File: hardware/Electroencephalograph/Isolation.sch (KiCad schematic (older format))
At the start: 17 parts, among them U4 THI3-0511, U5 ADUM2401BRWZ

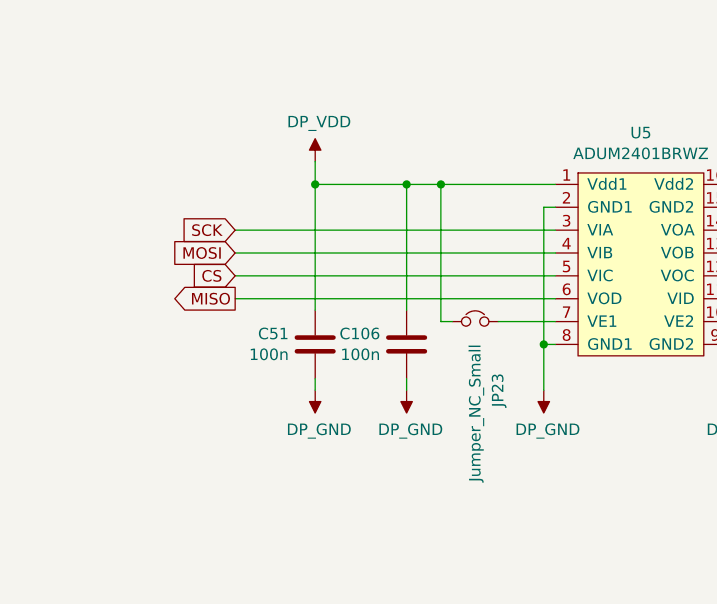
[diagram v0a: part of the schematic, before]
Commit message: further routing
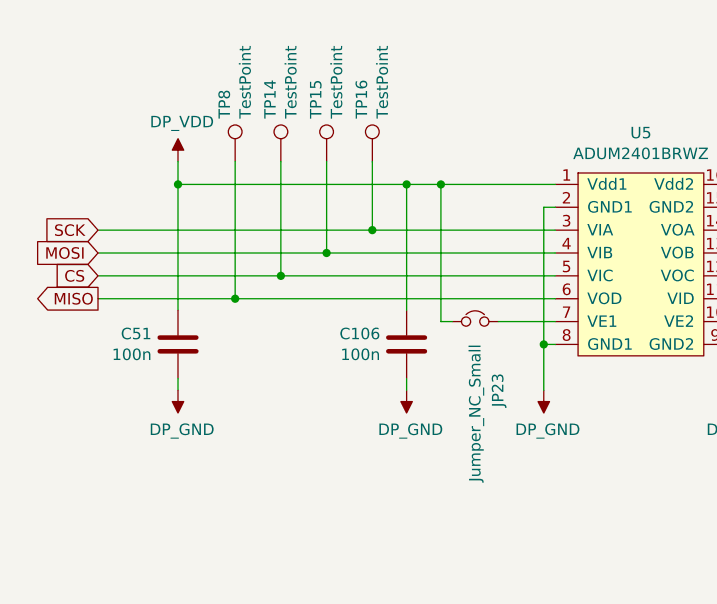
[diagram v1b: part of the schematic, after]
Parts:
- added TP14, TP15, TP16, TP8: TestPoint, TestPoint:TestPoint_Pad_D1.0mm, symbol Connector:TestPoint
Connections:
- net CS: now also TP14.1
- net MISO: now also TP8.1
- net MOSI: now also TP15.1
- net SCK: now also TP16.1
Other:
- moved on the sheet: C51
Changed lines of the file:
@@
 Wire Wire Line
 	3100 2600 3100 3200
-Text GLabel 1750 2700 0    50   Input ~ 0
+Text GLabel 1150 2700 0    50   Input ~ 0
 SCK
-Text GLabel 1750 2800 0    50   Input ~ 0
+Text GLabel 1150 2800 0    50   Input ~ 0
 MOSI
-Text GLabel 1750 2900 0    50   Input ~ 0
+Text GLabel 1150 2900 0    50   Input ~ 0
 CS
-Text GLabel 1750 3000 0    50   Output ~ 0
+Text GLabel 1150 3000 0    50   Output ~ 0
 MISO
 Wire Wire Line
-	3150 2700 1750 2700
-Wire Wire Line
-	3150 2800 1750 2800
-Wire Wire Line
-	3150 2900 1750 2900
-Wire Wire Line
-	3150 3000 1750 3000
-Connection ~ 2100 2500
-Wire Wire Line
-	2100 2500 2100 2400
-Wire Wire Line
-	2100 2500 2100 3050
+	3150 2700 2350 2700
+Wire Wire Line
+	3150 2800 2150 2800
+Wire Wire Line
+	3150 2900 1950 2900
+Connection ~ 1500 2500
+Wire Wire Line
+	1500 2500 1500 2400
+Wire Wire Line
+	1500 2500 1500 3050
 $Comp
 L Device:C C?
 U 1 1 5E028BA8
-P 2100 3200
+P 1500 3200
 AR Path="/5DF4CFF8/5E028BA8" Ref="C?"  Part="1"
 AR Path="/5DF61103/5E028BA8" Ref="C?"  Part="1"
 AR Path="/5DFE0AD6/5E028BA8" Ref="C51"  Part="1"
-F 0 "C51" H 2215 3246 50  0000 L CNN
-F 1 "100n" H 2215 3155 50  0000 L CNN
-F 2 "Capacitor_SMD:C_0402_1005Metric" H 2138 3050 50  0001 C CNN
-F 3 "~" H 2100 3200 50  0001 C CNN
-	1    2100 3200
+F 0 "C51" H 1615 3246 50  0000 L CNN
+F 1 "100n" H 1615 3155 50  0000 L CNN
+F 2 "Capacitor_SMD:C_0402_1005Metric" H 1538 3050 50  0001 C CNN
+F 3 "~" H 1500 3200 50  0001 C CNN
+	1    1500 3200
 	-1   0    0    -1
 $EndComp
@@
 L Electroencephalograph:DP_VDD #PWR101
 U 1 1 5E02F433
-P 2100 2400
-F 0 "#PWR101" H 2100 2525 50  0001 C CNN
-F 1 "DP_VDD" H 2117 2573 50  0000 C CNN
-F 2 "" H 2100 2525 50  0001 C CNN
-F 3 "" H 2100 2525 50  0001 C CNN
-	1    2100 2400
+P 1500 2400
+F 0 "#PWR101" H 1500 2525 50  0001 C CNN
+F 1 "DP_VDD" H 1517 2573 50  0000 C CNN
+F 2 "" H 1500 2525 50  0001 C CNN
+F 3 "" H 1500 2525 50  0001 C CNN
+	1    1500 2400
 	1    0    0    -1
 $EndComp
@@
 L Electroencephalograph:DP_GND #PWR102
 U 1 1 5E02EFAB
-P 2100 3400
-F 0 "#PWR102" H 2100 3425 50  0001 C CNN
-F 1 "DP_GND" H 2117 3227 50  0000 C CNN
-F 2 "" H 2100 3425 50  0001 C CNN
-F 3 "" H 2100 3425 50  0001 C CNN
-	1    2100 3400
+P 1500 3400
+F 0 "#PWR102" H 1500 3425 50  0001 C CNN
+F 1 "DP_GND" H 1517 3227 50  0000 C CNN
+F 2 "" H 1500 3425 50  0001 C CNN
+F 3 "" H 1500 3425 50  0001 C CNN
+	1    1500 3400
 	1    0    0    -1
 $EndComp
@@
 $EndComp
 Wire Wire Line
-	2100 3400 2100 3350
+	1500 3400 1500 3350
 Connection ~ 3100 3200
 Wire Wire Line
@@
 	2500 3050 2500 2500
 Wire Wire Line
-	2100 2500 2500 2500
+	1500 2500 2500 2500
 Connection ~ 2500 2500
 Wire Wire Line
@@
 Wire Wire Line
 	4650 2500 5050 2500
+$Comp
+L Connector:TestPoint TP?
+U 1 1 5E2E87E0
+P 2350 2400
+AR Path="/5DF61103/5E2E87E0" Ref="TP?"  Part="1"
+AR Path="/5E142744/5E2E87E0" Ref="TP?"  Part="1"
+AR Path="/5DFE0AD6/5E2E87E0" Ref="TP16"  Part="1"
+F 0 "TP16" V 2304 2588 50  0000 L CNN
+F 1 "TestPoint" V 2395 2588 50  0000 L CNN
+F 2 "TestPoint:TestPoint_Pad_D1.0mm" H 2550 2400 50  0001 C CNN
+F 3 "~" H 2550 2400 50  0001 C CNN
+	1    2350 2400
+	1    0    0    -1
+$EndComp
+$Comp
+L Connector:TestPoint TP?
+U 1 1 5E2E87E6
+P 2150 2400
+AR Path="/5DF61103/5E2E87E6" Ref="TP?"  Part="1"
+AR Path="/5E142744/5E2E87E6" Ref="TP?"  Part="1"
+AR Path="/5DFE0AD6/5E2E87E6" Ref="TP15"  Part="1"
+F 0 "TP15" V 2104 2588 50  0000 L CNN
+F 1 "TestPoint" V 2195 2588 50  0000 L CNN
+F 2 "TestPoint:TestPoint_Pad_D1.0mm" H 2350 2400 50  0001 C CNN
+F 3 "~" H 2350 2400 50  0001 C CNN
+	1    2150 2400
+	1    0    0    -1
+$EndComp
+$Comp
+L Connector:TestPoint TP?
+U 1 1 5E2E87EC
+P 1950 2400
+AR Path="/5DF61103/5E2E87EC" Ref="TP?"  Part="1"
+AR Path="/5E142744/5E2E87EC" Ref="TP?"  Part="1"
+AR Path="/5DFE0AD6/5E2E87EC" Ref="TP14"  Part="1"
+F 0 "TP14" V 1904 2588 50  0000 L CNN
+F 1 "TestPoint" V 1995 2588 50  0000 L CNN
+F 2 "TestPoint:TestPoint_Pad_D1.0mm" H 2150 2400 50  0001 C CNN
+F 3 "~" H 2150 2400 50  0001 C CNN
+	1    1950 2400
+	1    0    0    -1
+$EndComp
+$Comp
+L Connector:TestPoint TP?
+U 1 1 5E2E87F2
+P 1750 2400
+AR Path="/5DF61103/5E2E87F2" Ref="TP?"  Part="1"
+AR Path="/5E142744/5E2E87F2" Ref="TP?"  Part="1"
+AR Path="/5DFE0AD6/5E2E87F2" Ref="TP8"  Part="1"
+F 0 "TP8" V 1704 2588 50  0000 L CNN
+F 1 "TestPoint" V 1795 2588 50  0000 L CNN
+F 2 "TestPoint:TestPoint_Pad_D1.0mm" H 1950 2400 50  0001 C CNN
+F 3 "~" H 1950 2400 50  0001 C CNN
+	1    1750 2400
+	1    0    0    -1
+$EndComp
+Wire Wire Line
+	2350 2400 2350 2700
+Connection ~ 2350 2700
+Wire Wire Line
+	2350 2700 1150 2700
+Wire Wire Line
+	2150 2400 2150 2800
+Connection ~ 2150 2800
+Wire Wire Line
+	2150 2800 1150 2800
+Wire Wire Line
+	1950 2400 1950 2900
+Connection ~ 1950 2900
+Wire Wire Line
+	1950 2900 1150 2900
+Wire Wire Line
+	1750 2400 1750 3000
+Wire Wire Line
+	1150 3000 1750 3000
+Connection ~ 1750 3000
+Wire Wire Line
+	1750 3000 3150 3000
 $EndSCHEMATC
